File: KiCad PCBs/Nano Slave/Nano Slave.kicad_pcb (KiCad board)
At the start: 2 copper layers, 80 x 55.9 mm, 49 parts, among them J1 Screw_Terminal_01x02, J10 AVR-ISP-6, J11 Conn_01x06_Female, J12 Screw_Terminal_01x02, J13 Screw_Terminal_01x02, J14 Screw_Terminal_01x02, J15 Screw_Terminal_01x02, J16 Screw_Terminal_01x02, J2 Screw_Terminal_01x02, J3 Screw_Terminal_01x02, J4 Screw_Terminal_01x02, J5 Screw_Terminal_01x02, J6 Screw_Terminal_01x02, J7 Screw_Terminal_01x02, J8 Screw_Terminal_01x02, J9 Screw_Terminal_01x02, SW1 SW_DIP_x02, SW2 SW_DIP_x02, SW3 SW_MEC_5E, U1 ATmega328P-AU, U2 MAX487ESA+T, U3 ULN2003A, U5 AMS1117-5.0, Y1 Crystal_GND24

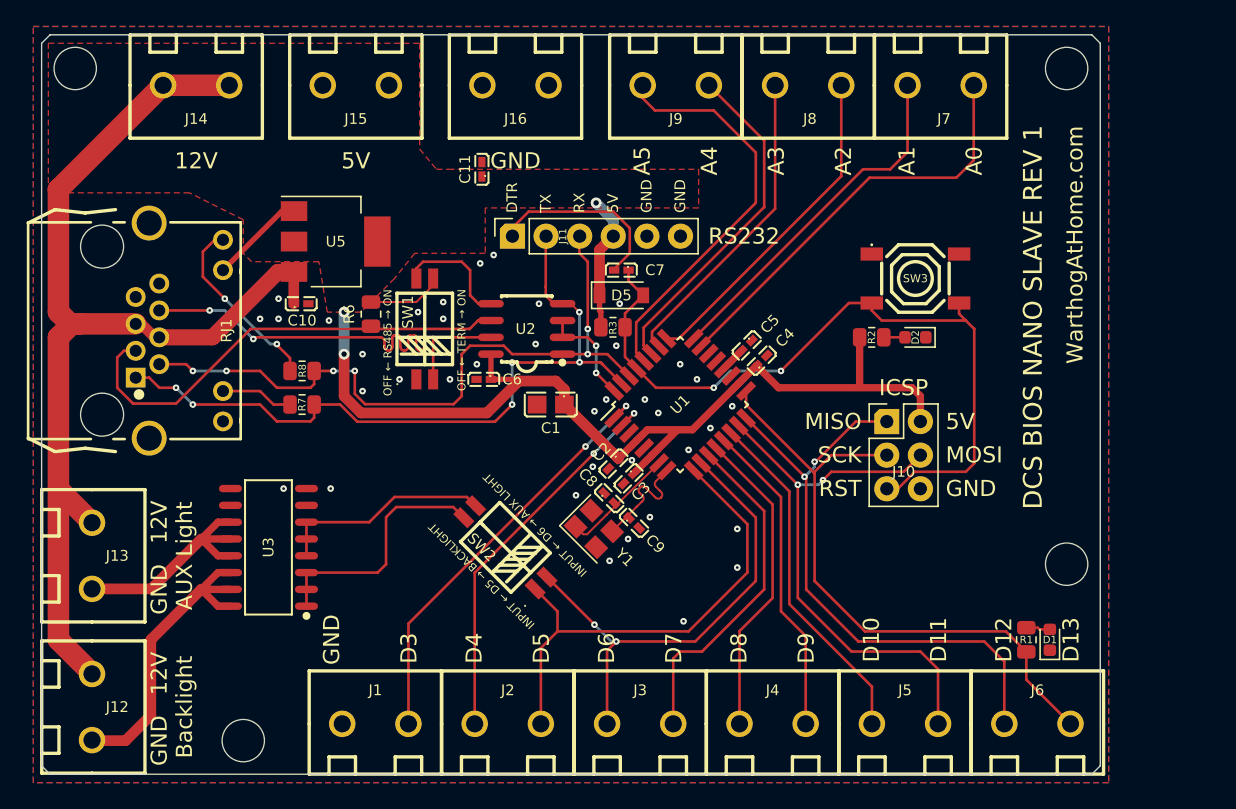
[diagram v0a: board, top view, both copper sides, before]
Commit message: Nano Slave Rev 2
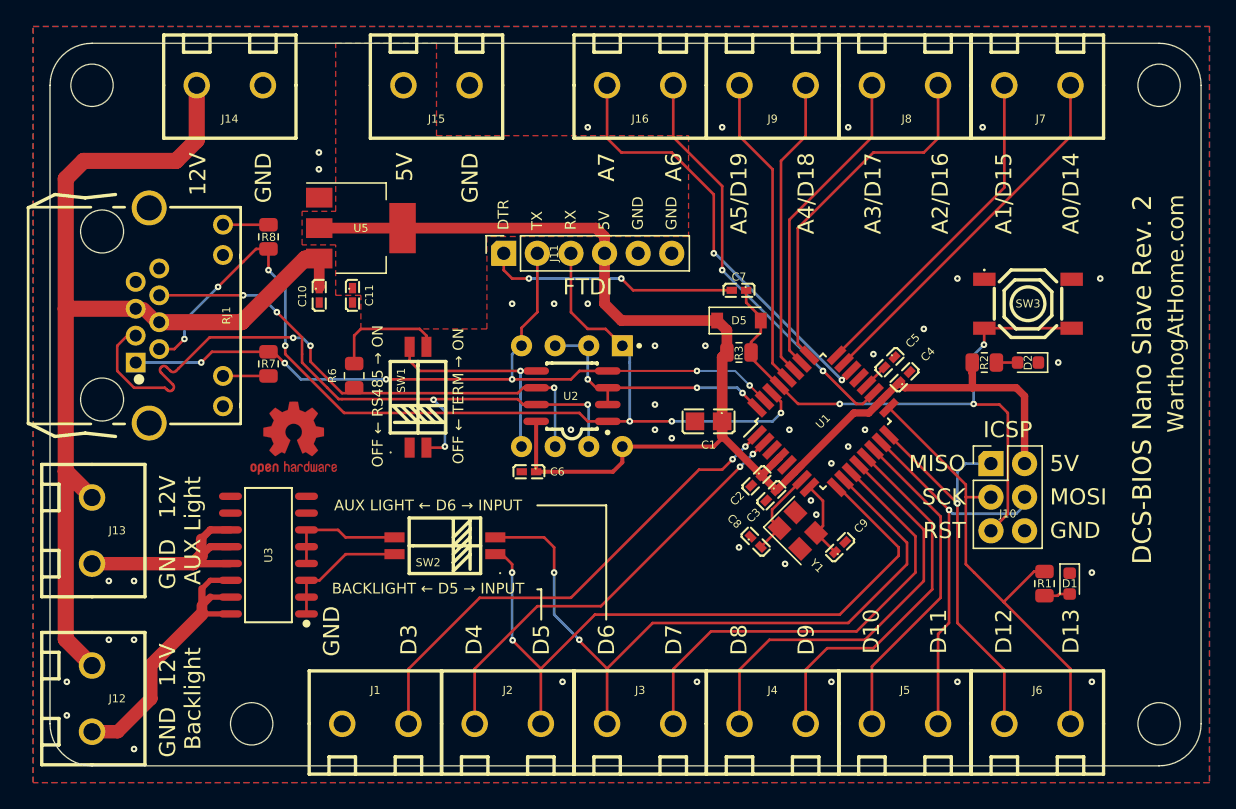
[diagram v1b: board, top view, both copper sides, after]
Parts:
- added REF**: OSHW-Logo2_7.3x6mm_Copper, Symbol:OSHW-Logo2_7.3x6mm_Copper, F.Cu at (120.7, 106.7)
- added U4: MAX487CPA+, Package_DIP:DIP-8_W7.62mm, F.Cu at (145.5, 99.7)
- moved C9 15.7 mm to (161.9, 114.9), turned to 45 degrees
- moved Y1 15.4 mm to (158.8, 113.7)
- moved H4 13.9 mm to (186.1, 128.3)
- moved C11 13.7 mm to (125.1, 95.9), turned to -90 degrees
- moved C1 12.0 mm to (152.0, 105.4)
- moved C8 11.5 mm to (155.6, 114.5)
- moved C2 10.9 mm to (155.6, 109.9)
- moved U1 10.9 mm to (160.7, 105.4)
- moved C5 10.9 mm to (165.7, 100.9)
- moved C4 10.9 mm to (166.8, 102.1)
- moved C3 10.9 mm to (156.7, 111.0)
- moved R8 10.4 mm to (118.7, 91.5), turned to -90 degrees
- moved R3 9.71 mm to (154.3, 100.2)
- moved J16 9.42 mm to (146.8, 80.0)
- moved D5 9.09 mm to (154.3, 97.8)
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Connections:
- J14 pad 1: +12V -> GND
- J15 pad 1: +5V -> GND
- J16 pad 1: GND -> A6
- J16 pad 2: GND -> A7
- U1 pad 19: unconnected-(U1-Pad19) -> A6
- U1 pad 22: unconnected-(U1-Pad22) -> A7
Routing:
- net A7: track 0.00 -> 33.0 mm, vias 0 -> 2
- net A6: track 0.00 -> 31.5 mm, vias 0 -> 2
- net RXD: track 52.6 -> 77.6 mm, vias 6 -> 7
- net +5V: track 83.1 -> 102.1 mm, vias 3 -> 0
- net D6: track 36.8 -> 54.0 mm
- net D5: track 37.0 -> 52.3 mm, vias 0 -> 2
- net D12: track 44.9 -> 30.6 mm, vias 2 -> 1
- net RS485+: track 35.3 -> 48.6 mm, vias 0 -> 3
- net D13: track 47.6 -> 35.5 mm
- net D2: track 8.06 -> 20.1 mm, vias 2 -> 3
- net D11: track 42.0 -> 30.4 mm, vias 2 -> 1
- net RS485-: track 34.3 -> 45.4 mm, vias 2 -> 5
- net Net-(R8-Pad1): track 13.9 -> 3.44 mm, vias 2 -> 0
- net D7: track 25.8 -> 35.0 mm
- net BACKLIGHT_BASE: track 18.9 -> 10.0 mm
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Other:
- board size 80 x 55.9 mm -> 87 x 54.6 mm
- board text added: "${TITLE} Rev. ${REVISION}"
- board text added: "AUX LIGHT ← D6 → INPUT"
- board text added: "BACKLIGHT ← D5 → INPUT"
- board text removed: "DCS BIOS NANO SLAVE REV 1"
- board text removed: "INPUT ← D5 → BACKLIGHT"
- board text removed: "INPUT ← D6 → AUX LIGHT"
